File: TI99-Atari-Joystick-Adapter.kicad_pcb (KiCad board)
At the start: 2 copper layers, 13 parts, among them J1 DE9_Plug_MountingHoles, J2 DE9_Plug_MountingHoles, J3 DE9_Receptacle_MountingHoles

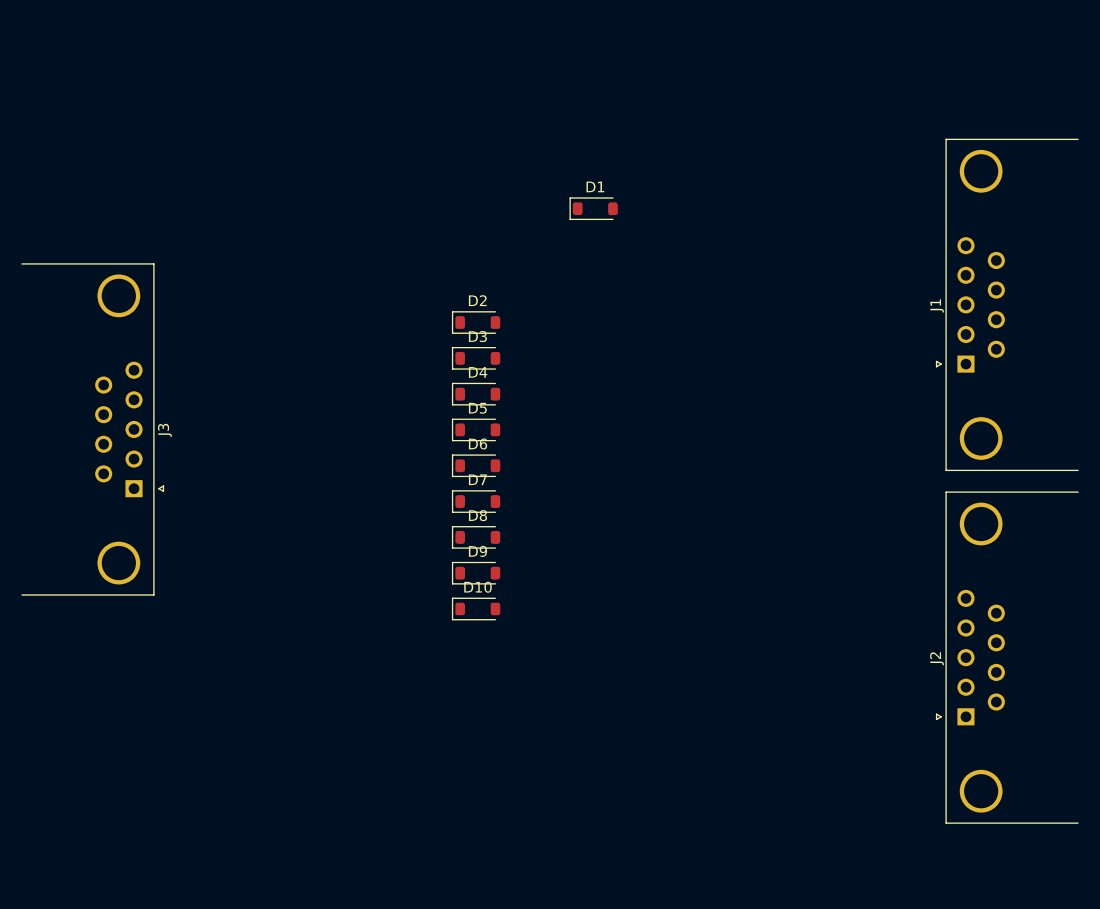
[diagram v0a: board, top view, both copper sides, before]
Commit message: Initial Design v0.01
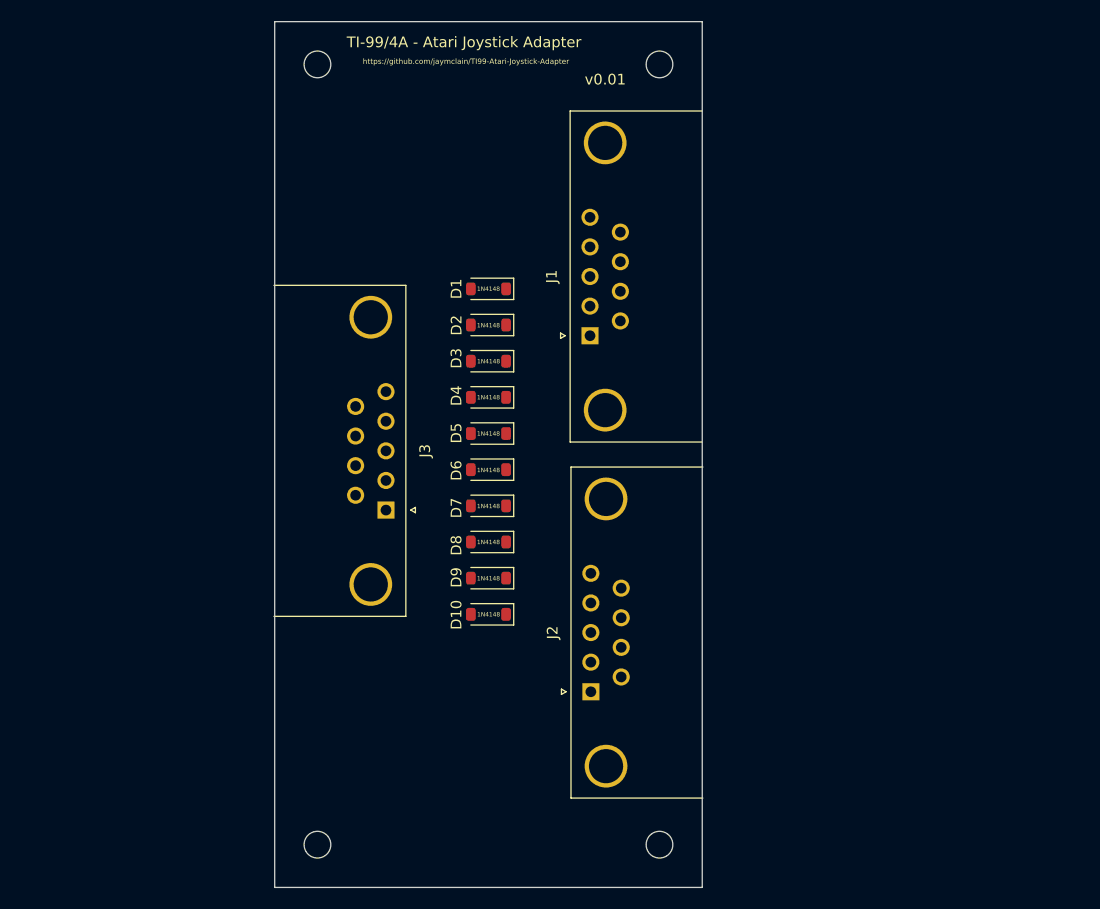
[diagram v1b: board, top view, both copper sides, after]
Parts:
- added H1: MountingHole, MountingHole:MountingHole_2.5mm, F.Cu at (129.0, 59.0)
- added H2: MountingHole, MountingHole:MountingHole_2.5mm, F.Cu at (161.0, 59.0)
- added H3: MountingHole, MountingHole:MountingHole_2.5mm, F.Cu at (129.0, 132.0)
- added H4: MountingHole, MountingHole:MountingHole_2.5mm, F.Cu at (161.0, 132.0)
- D1, D10, D2, D3, D4, D5, D6, D7, D8, D9: value 1N4148W -> 1N4148
- moved J1 35.3 mm to (154.5, 84.4)
- moved J2 35.2 mm to (154.6, 117.7)
- moved J3 23.7 mm to (135.4, 100.7)
- moved D1 12.5 mm to (145.0, 80.0), turned to 180 degrees
- moved D10 1.12 mm to (145.0, 110.5), turned to 180 degrees
- moved D9 1.10 mm to (145.0, 107.1), turned to 180 degrees
- moved D8 1.09 mm to (145.0, 103.7), turned to 180 degrees
- moved D7 1.08 mm to (145.0, 100.3), turned to 180 degrees
- moved D6 1.07 mm to (145.0, 96.9), turned to 180 degrees
- moved D5 1.05 mm to (145.0, 93.5), turned to 180 degrees
- moved D4 1.04 mm to (145.0, 90.2), turned to 180 degrees
- moved D3 1.03 mm to (145.0, 86.8), turned to 180 degrees
- moved D2 1.03 mm to (145.0, 83.4), turned to 180 degrees
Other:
- board outline added: 40 x 81 mm
- board text added: "TI-99/4A - Atari Joystick Adapter"
- board text added: "https://github.com/jaymclain/TI99-Atari-Joystick-Adapter"
- board text added: "v0.01"
